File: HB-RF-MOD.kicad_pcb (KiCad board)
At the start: 2 copper layers, 35.6 x 64.2 mm, 25 parts, among them J1 RPi Header, J2 RGB, Q1 BC847, SW1 Button, U1 TRX2-TIF, U2 RX8130-CE, U3 3V3LDO

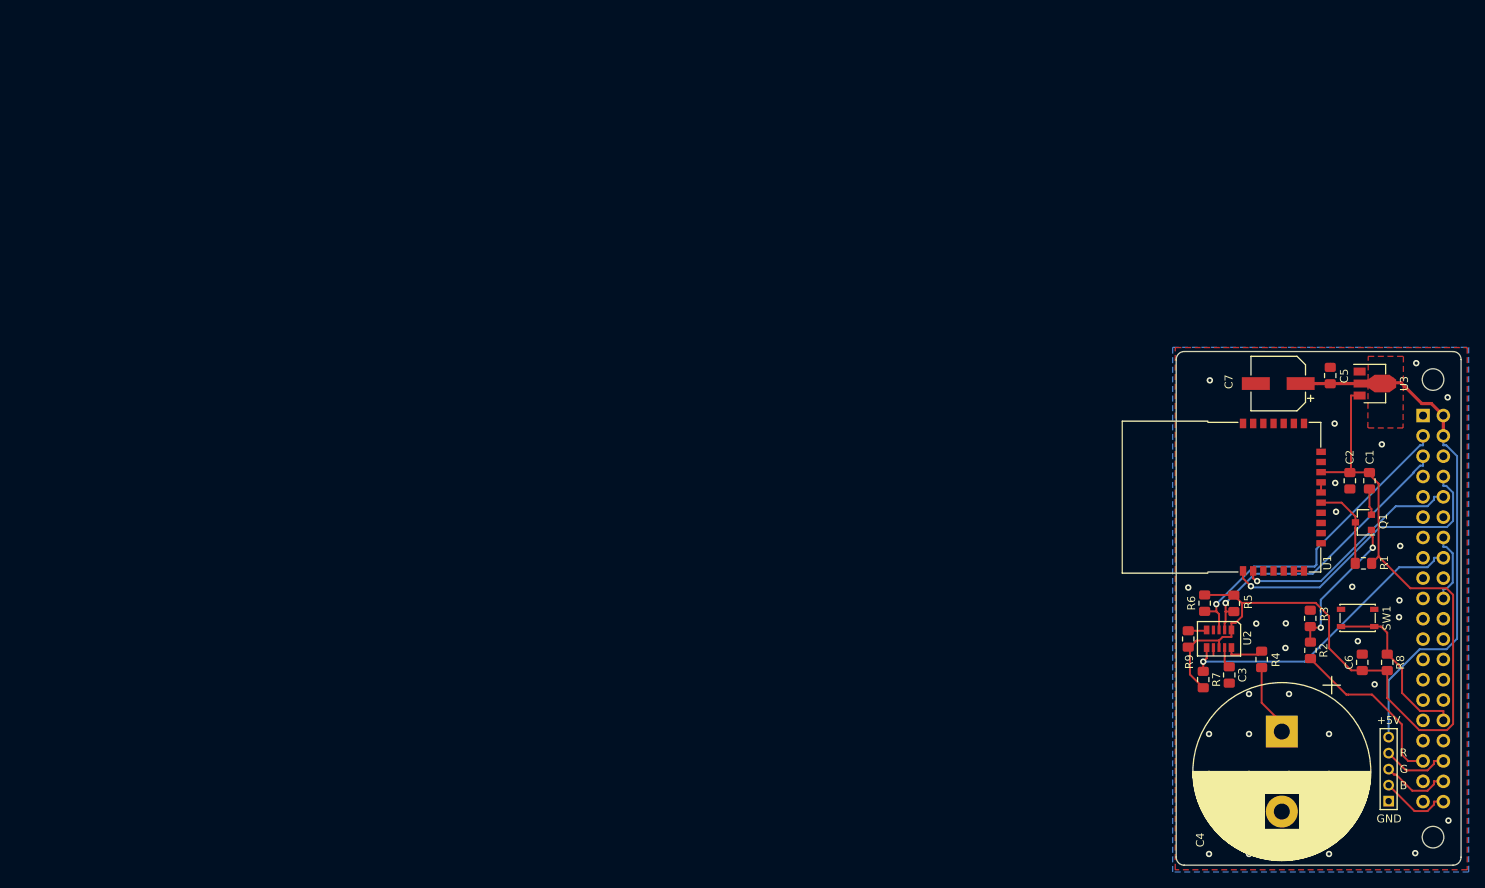
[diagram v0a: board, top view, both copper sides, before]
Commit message: update
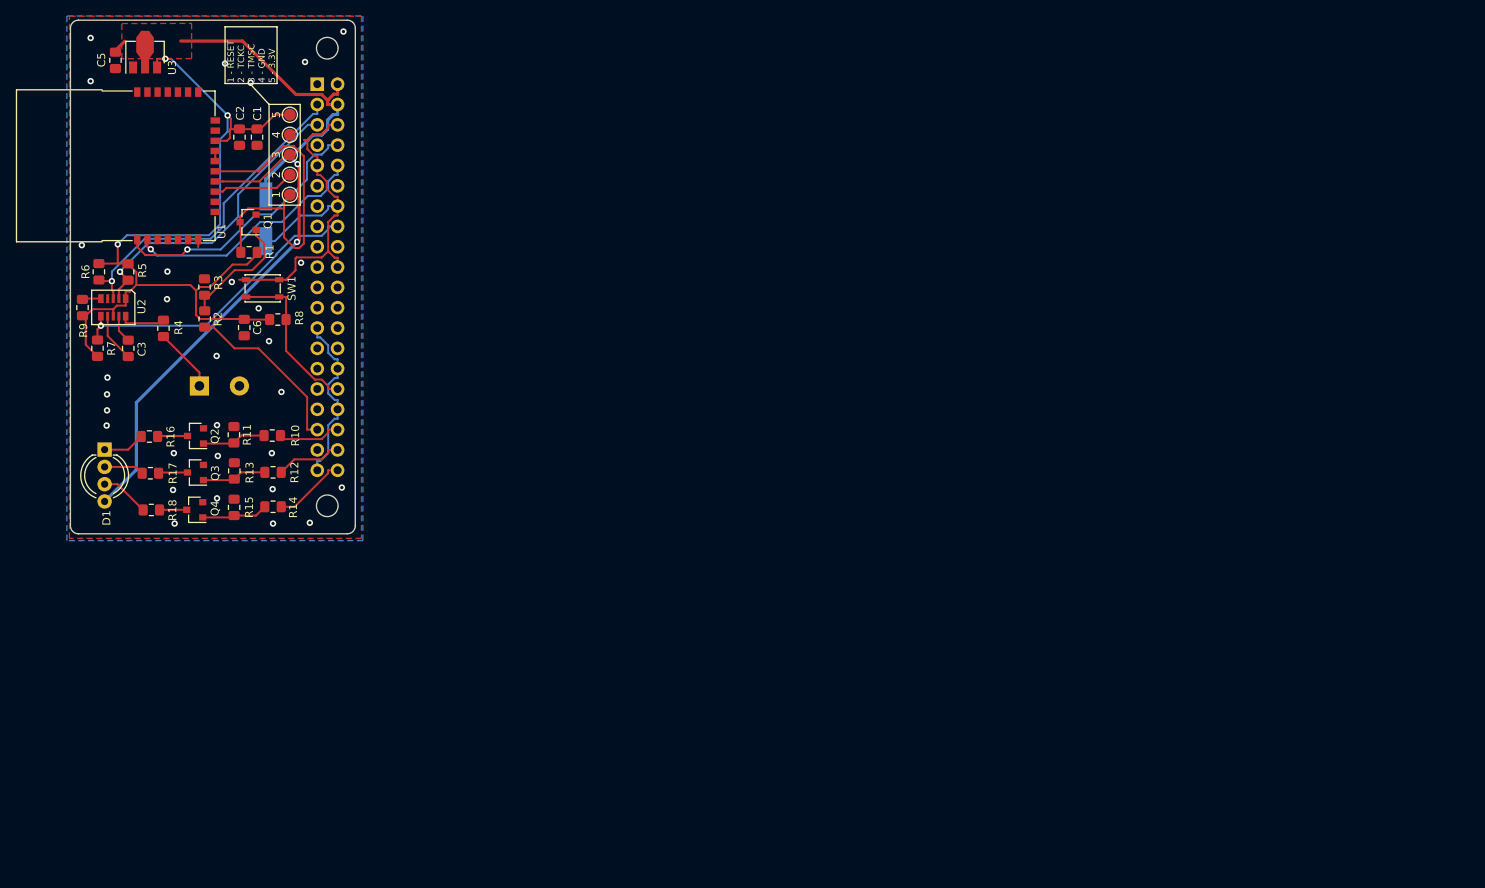
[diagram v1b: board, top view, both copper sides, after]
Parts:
- added D1: LED_RGBA, LED_THT:LED_D5.0mm-4_RGB_Wide_Pins, F.Cu at (26.9, 69.5)
- added J3: GND, TestPoint:TestPoint_Pad_D1.5mm, F.Cu at (50.1, 30.1)
- added J4: RESET, TestPoint:TestPoint_Pad_D1.5mm, F.Cu at (50.1, 37.6)
- added J5: J_TCKC, TestPoint:TestPoint_Pad_D1.5mm, F.Cu at (50.1, 35.1)
- added J6: J_TMSC, TestPoint:TestPoint_Pad_D1.5mm, F.Cu at (50.1, 32.6)
- added Q2: BC847, Package_TO_SOT_SMD:SOT-23, F.Cu at (38.3, 67.8)
- added Q3: BC847, Package_TO_SOT_SMD:SOT-23, F.Cu at (38.3, 72.3)
- added Q4: BC847, Package_TO_SOT_SMD:SOT-23, F.Cu at (38.2, 77.0)
- added R10: 10k, Resistor_SMD:R_0805_2012Metric_Pad1.15x1.40mm_HandSolder, F.Cu at (47.9, 67.7)
- added R11: 10k, Resistor_SMD:R_0805_2012Metric_Pad1.15x1.40mm_HandSolder, F.Cu at (43.1, 67.6)
- added R12: 10k, Resistor_SMD:R_0805_2012Metric_Pad1.15x1.40mm_HandSolder, F.Cu at (48.0, 72.3)
- added R13: 10k, Resistor_SMD:R_0805_2012Metric_Pad1.15x1.40mm_HandSolder, F.Cu at (43.2, 72.1)
- added R14: 10k, Resistor_SMD:R_0805_2012Metric_Pad1.15x1.40mm_HandSolder, F.Cu at (48.0, 76.6)
- added R15: 10k, Resistor_SMD:R_0805_2012Metric_Pad1.15x1.40mm_HandSolder, F.Cu at (43.1, 76.7)
- added R16: 180, Resistor_SMD:R_0805_2012Metric_Pad1.15x1.40mm_HandSolder, F.Cu at (32.5, 67.8)
- added R17: 100, Resistor_SMD:R_0805_2012Metric_Pad1.15x1.40mm_HandSolder, F.Cu at (32.7, 72.4)
- added R18: 100, Resistor_SMD:R_0805_2012Metric_Pad1.15x1.40mm_HandSolder, F.Cu at (32.8, 77.0)
- C4: footprint Capacitor_THT:CP_Radial_D22.0mm_P10.00mm_SnapIn -> additional:CP_Radial_D20.0mm_P5.00mm; moved to B.Cu
- C7: moved to B.Cu
- J2: value RGB -> 3V3; footprint Connector_PinHeader_2.00mm:PinHeader_1x05_P2.00mm_Vertical -> TestPoint:TestPoint_Pad_D1.5mm
- moved J2 161.9 mm to (50.1, 27.6), turned to 0 degrees
- moved U3 158.7 mm to (32.0, 20.2), turned to 90 degrees
- moved C5 156.9 mm to (28.3, 20.8), turned to 270 degrees
- moved C6 145.9 mm to (44.4, 54.2), turned to 270 degrees
- moved C1 145.5 mm to (46.0, 30.4)
- moved C2 145.3 mm to (43.8, 30.4)
- moved R8 145.1 mm to (48.6, 53.2), turned to 180 degrees
- moved R1 144.6 mm to (45.0, 44.8)
- moved Q1 144.4 mm to (44.9, 41.0)
- moved R2 144.3 mm to (39.5, 53.1)
- moved H1 144.3 mm to (54.8, 76.5)
- moved H2 144.3 mm to (54.8, 19.3)
- moved J1 144.3 mm to (53.5, 23.8)
- moved R3 144.3 mm to (39.4, 49.1)
- moved R5 144.3 mm to (29.9, 47.3)
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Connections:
- J1 pad 36: Net-(J1-Pad36) -> RGB-RED
- J1 pad 38: Net-(J1-Pad38) -> RGB-GREEN
- J1 pad 40: Net-(J1-Pad40) -> RGB-BLUE
- J2 pad 1: GND -> +3V3
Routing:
- net GND: track 16.0 -> 82.6 mm, vias 34 -> 30
- net +5V: track 65.9 -> 99.0 mm, vias 0 -> 2
- net Net-(J4-Pad1): track 10.9 -> 43.1 mm
- net Net-(J6-Pad1): track 0.00 -> 10.7 mm
- net Net-(J5-Pad1): track 0.00 -> 10.2 mm
- net RGB-BLUE: track 0.00 -> 9.15 mm
- net Net-(J1-Pad40): track 8.88 -> 0.00 mm
- net Net-(J1-Pad38): track 8.66 -> 0.00 mm
- net Net-(J1-Pad36): track 8.43 -> 0.00 mm
- net RGB-GREEN: track 0.00 -> 8.42 mm
- net Net-(Q4-Pad1): track 0.00 -> 8.32 mm
- net Net-(Q3-Pad1): track 0.00 -> 8.08 mm
- net RGB-RED: track 0.00 -> 8.04 mm
- net Net-(Q2-Pad1): track 0.00 -> 7.98 mm
- net +3V3: track 117.0 -> 109.1 mm, vias 0 -> 3
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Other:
- net class 5V added: clearance 0.2, trace_width 0.4, via_dia 0.8, via_drill 0.4
- board text added: "1"
- board text added: "1 - RESET 2 - TCKC 3 - TMSC 4 - GND 5 - 3.3V"
- board text added: "2"
- board text added: "3"
- board text added: "4"
- board text added: "5"
- board text removed: "+5V"
- board text removed: "B"
- board text removed: "G"
- board text removed: "GND"
- board text removed: "R"
